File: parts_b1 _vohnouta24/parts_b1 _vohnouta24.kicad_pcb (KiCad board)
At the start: 2 copper layers, 2 parts, among them J1 encoder, J2 SIMSD

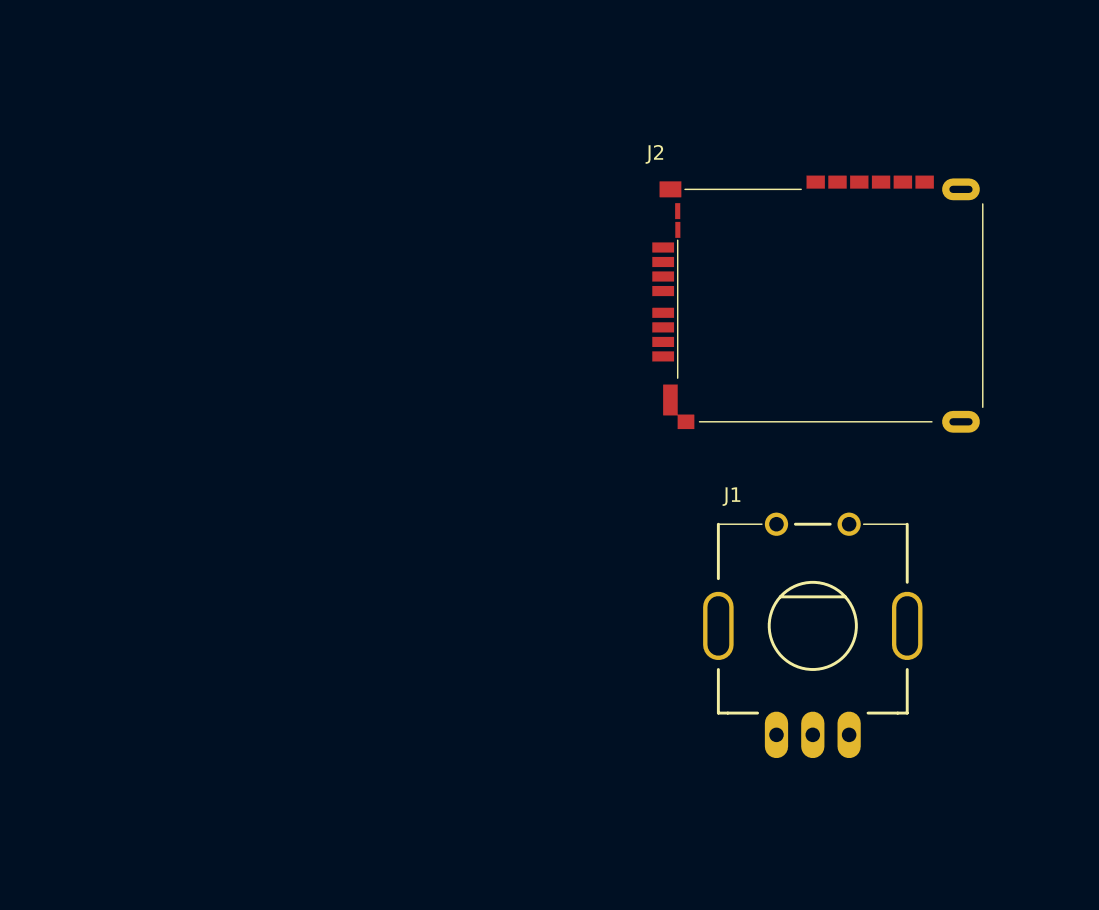
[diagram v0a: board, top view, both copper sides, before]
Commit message: Fix
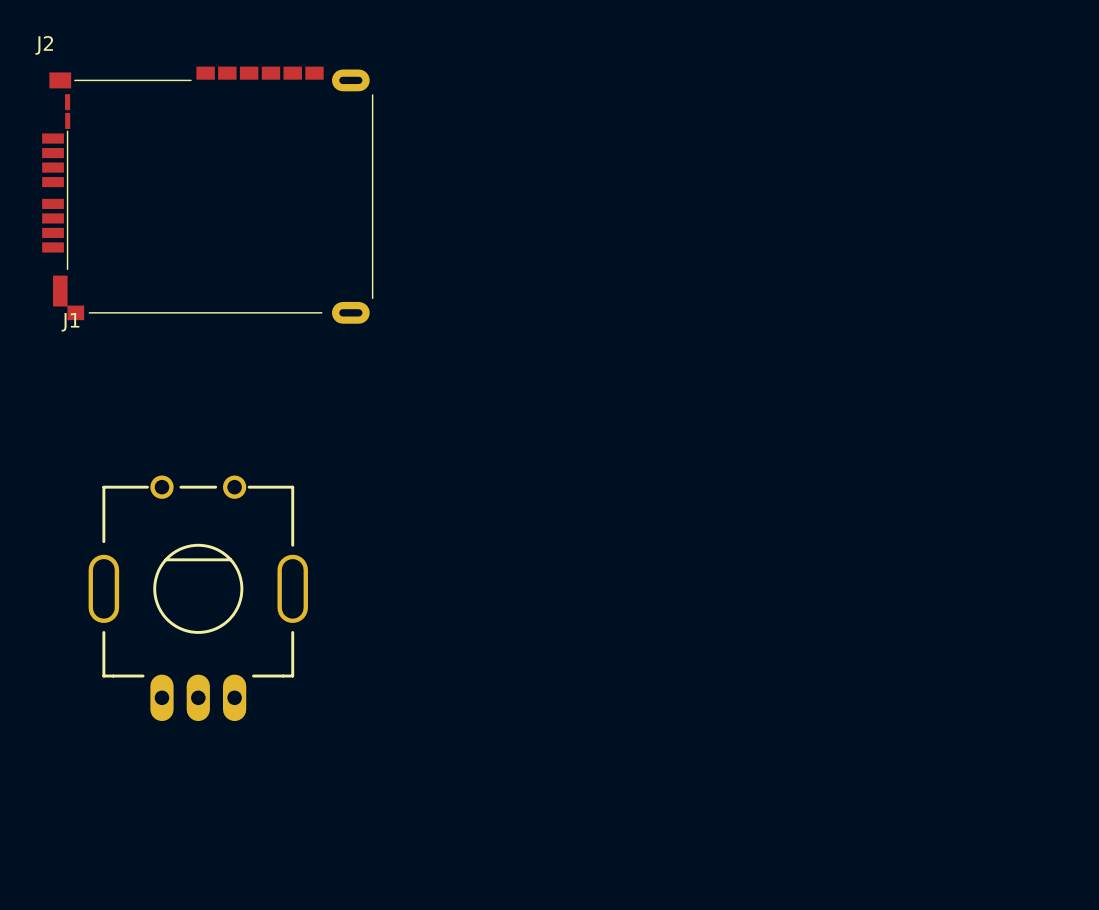
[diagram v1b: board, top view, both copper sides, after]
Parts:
- moved J2 42.7 mm to (127.5, 75.5)
- moved J1 42.4 mm to (129.0, 103.0)
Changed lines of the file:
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@@
 	(footprint "parts_b1_vohnouta24:encoder"
 		(layer "F.Cu")
-		(at 171.3 105.55)
+		(at 129 103)
 		(property "Reference" "J1"
-			(at -5.5 -9 0)
+			(at -8.7 -18.45 0)
 			(unlocked yes)
 			(layer "F.SilkS")
@@
 		)
 		(property "Value" "encoder"
-			(at 4.5 -9 0)
+			(at 1.3 -18.45 0)
 			(unlocked yes)
 			(layer "F.Fab")
@@
 			(end -3.5 -7)
 			(stroke
-				(width 0.1)
-				(type default)
+				(width 0.2)
+				(type solid)
 			)
 			(layer "F.SilkS")
@@
 			(end 3.5 -7)
 			(stroke
-				(width 0.1)
-				(type default)
+				(width 0.2)
+				(type solid)
 			)
 			(layer "F.SilkS")
@@
 	(footprint "parts_b1_vohnouta24:SIMSD"
 		(layer "F.Cu")
-		(at 169.5 83)
+		(at 127.5 75.5)
 		(property "Reference" "J2"
 			(at -9 -10 0)

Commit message: bub fix (yes)
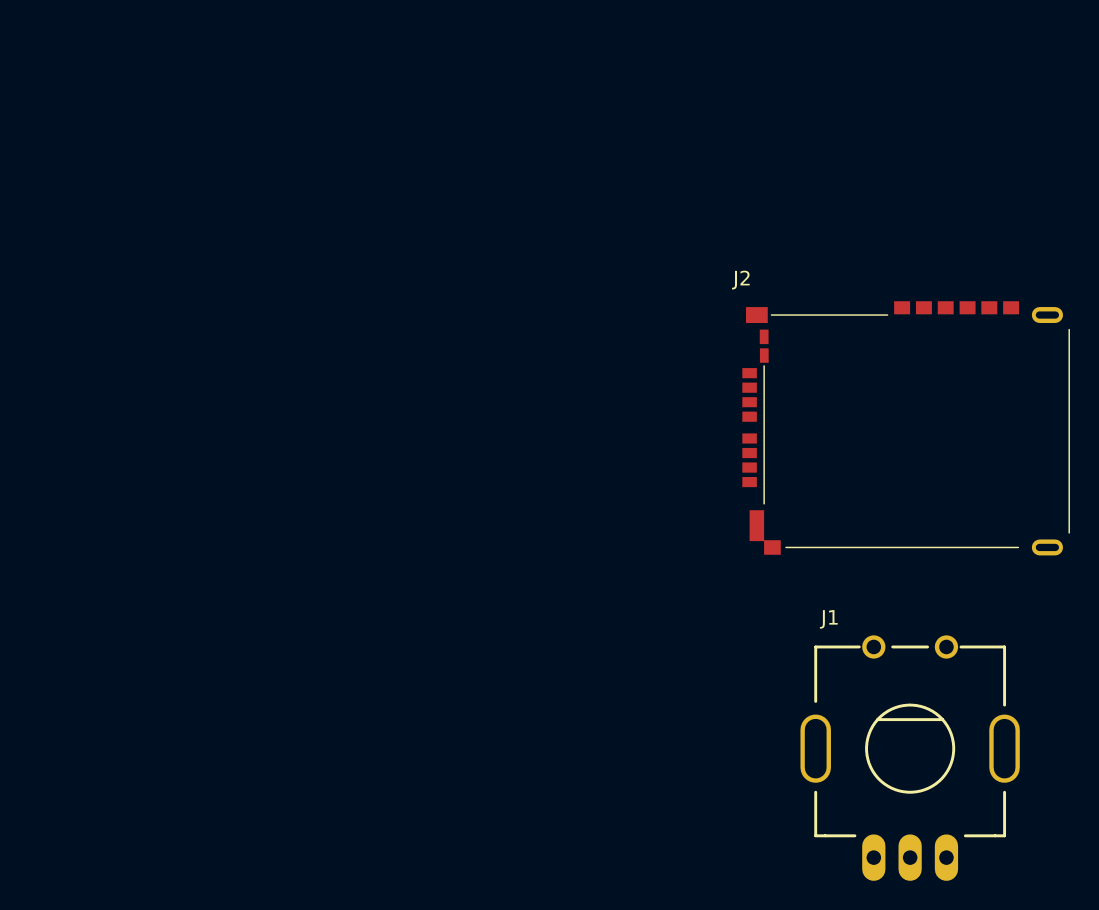
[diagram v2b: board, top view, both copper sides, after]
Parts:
- moved J2 50.6 mm to (175.4, 91.7)
- moved J1 50.2 mm to (178.0, 114.0)
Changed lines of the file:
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@@
 	)
 	(net 0 "")
-	(net 1 "unconnected-(J1-C-Pad3)")
-	(net 2 "unconnected-(J1-A-Pad1)")
+	(net 1 "unconnected-(J1-A-Pad1)")
+	(net 2 "unconnected-(J1-C-Pad3)")
 	(net 3 "unconnected-(J1-B-Pad2)")
-	(net 4 "unconnected-(J2-DAT1-Pad8)")
-	(net 5 "unconnected-(J2-VSS-Pad6)")
-	(net 6 "unconnected-(J2-VCC-Pad11)")
-	(net 7 "unconnected-(J2-DAT3-Pad2)")
-	(net 8 "unconnected-(J2-IO-Pad16)")
-	(net 9 "unconnected-(J2-GND-Pad14)")
+	(net 4 "unconnected-(J2-IO-Pad16)")
+	(net 5 "unconnected-(J2-SWITCHA-Pad9)")
+	(net 6 "unconnected-(J2-DAT2-Pad1)")
+	(net 7 "unconnected-(J2-VSS-Pad6)")
+	(net 8 "unconnected-(J2-RST-Pad12)")
+	(net 9 "unconnected-(J2-CLK-Pad13)")
 	(net 10 "unconnected-(J2-CLK-Pad5)")
-	(net 11 "unconnected-(J2-VPP-Pad15)")
-	(net 12 "unconnected-(J2-CLK-Pad13)")
-	(net 13 "unconnected-(J2-DAT2-Pad1)")
-	(net 14 "unconnected-(J2-SWITCHA-Pad9)")
-	(net 15 "unconnected-(J2-VDD-Pad4)")
-	(net 16 "unconnected-(J2-CMD-Pad3)")
-	(net 17 "unconnected-(J2-SWITCHB-Pad10)")
-	(net 18 "unconnected-(J2-DAT0-Pad7)")
-	(net 19 "unconnected-(J2-RST-Pad12)")
+	(net 11 "unconnected-(J2-DAT0-Pad7)")
+	(net 12 "unconnected-(J2-VCC-Pad11)")
+	(net 13 "unconnected-(J2-CMD-Pad3)")
+	(net 14 "unconnected-(J2-DAT3-Pad2)")
+	(net 15 "unconnected-(J2-GND-Pad14)")
+	(net 16 "unconnected-(J2-SWITCHB-Pad10)")
+	(net 17 "unconnected-(J2-VPP-Pad15)")
+	(net 18 "unconnected-(J2-VDD-Pad4)")
+	(net 19 "unconnected-(J2-DAT1-Pad8)")
 	(footprint "parts_b1_vohnouta24:encoder"
 		(layer "F.Cu")
-		(at 129 103)
+		(at 178 114)
 		(property "Reference" "J1"
-			(at -8.7 -18.45 0)
+			(at -5.5 -9 0)
 			(unlocked yes)
 			(layer "F.SilkS")
@@
 		)
 		(property "Value" "encoder"
-			(at 1.3 -18.45 0)
+			(at 4.5 -9 0)
 			(unlocked yes)
 			(layer "F.Fab")
@@
 			(layers "*.Cu" "*.Mask")
 			(remove_unused_layers no)
-			(net 2 "unconnected-(J1-A-Pad1)")
+			(net 1 "unconnected-(J1-A-Pad1)")
 			(pinfunction "A")
 			(pintype "passive")
@@
 			(layers "*.Cu" "*.Mask")
 			(remove_unused_layers no)
-			(net 1 "unconnected-(J1-C-Pad3)")
+			(net 2 "unconnected-(J1-C-Pad3)")
 			(pinfunction "C")
 			(pintype "passive")
@@
 	(footprint "parts_b1_vohnouta24:SIMSD"
 		(layer "F.Cu")
-		(at 127.5 75.5)
+		(at 175.45 91.65)
 		(property "Reference" "J2"
 			(at -9 -10 0)
@@
 		)
 		(property "Value" "SIMSD"
-			(at -7.5 11 0)
+			(at -3.5 15.5 0)
 			(unlocked yes)
 			(layer "F.Fab")
@@
 			(layer "F.SilkS")
 		)
+		(pad "" smd rect
+			(at -8 -7.5)
+			(size 1.5 1.1)
+			(layers "F.Cu" "F.Mask" "F.Paste")
+		)
+		(pad "" smd rect
+			(at -8 7)
+			(size 1 2.13)
+			(layers "F.Cu" "F.Mask" "F.Paste")
+		)
+		(pad "" smd rect
+			(at -6.93 8.5)
+			(size 1.15 1)
+			(layers "F.Cu" "F.Mask" "F.Paste")
+		)
+		(pad "" thru_hole oval
+			(at 12 -7.5)
+			(size 2.15 1.1)
+			(drill oval 1.6 0.5)
+			(layers "*.Cu" "*.Mask")
+			(remove_unused_layers no)
+		)
+		(pad "" thru_hole oval
+			(at 12 8.5)
+			(size 2.15 1.1)
+			(drill oval 1.6 0.5)
+			(layers "*.Cu" "*.Mask")
+			(remove_unused_layers no)
+		)
 		(pad "1" smd rect
 			(at -8.5 -3.5 180)
-			(size 1.5 0.7)
-			(layers "F.Cu" "F.Mask" "F.Paste")
-			(net 13 "unconnected-(J2-DAT2-Pad1)")
+			(size 1 0.7)
+			(layers "F.Cu" "F.Mask" "F.Paste")
+			(net 6 "unconnected-(J2-DAT2-Pad1)")
 			(pinfunction "DAT2")
 			(pintype "bidirectional")
@@
 		(pad "2" smd rect
 			(at -8.5 -2.5 180)
-			(size 1.5 0.7)
-			(layers "F.Cu" "F.Mask" "F.Paste")
-			(net 7 "unconnected-(J2-DAT3-Pad2)")
+			(size 1 0.7)
+			(layers "F.Cu" "F.Mask" "F.Paste")
+			(net 14 "unconnected-(J2-DAT3-Pad2)")
 			(pinfunction "DAT3")
 			(pintype "bidirectional")
@@
 		(pad "3" smd rect
 			(at -8.5 -1.5 180)
-			(size 1.5 0.7)
-			(layers "F.Cu" "F.Mask" "F.Paste")
-			(net 16 "unconnected-(J2-CMD-Pad3)")
+			(size 1 0.7)
+			(layers "F.Cu" "F.Mask" "F.Paste")
+			(net 13 "unconnected-(J2-CMD-Pad3)")
 			(pinfunction "CMD")
 			(pintype "bidirectional")
@@
 		(pad "4" smd rect
 			(at -8.5 -0.5 180)
-			(size 1.5 0.7)
-			(layers "F.Cu" "F.Mask" "F.Paste")
-			(net 15 "unconnected-(J2-VDD-Pad4)")
+			(size 1 0.7)
+			(layers "F.Cu" "F.Mask" "F.Paste")
+			(net 18 "unconnected-(J2-VDD-Pad4)")
 			(pinfunction "VDD")
 			(pintype "power_in")
@@
 		(pad "5" smd rect
 			(at -8.5 1 180)
-			(size 1.5 0.7)
+			(size 1 0.7)
 			(layers "F.Cu" "F.Mask" "F.Paste")
 			(net 10 "unconnected-(J2-CLK-Pad5)")
@@
 		(pad "6" smd rect
 			(at -8.5 2 180)
-			(size 1.5 0.7)
-			(layers "F.Cu" "F.Mask" "F.Paste")
-			(net 5 "unconnected-(J2-VSS-Pad6)")
+			(size 1 0.7)
+			(layers "F.Cu" "F.Mask" "F.Paste")
+			(net 7 "unconnected-(J2-VSS-Pad6)")
 			(pinfunction "VSS")
 			(pintype "power_in")
@@
 		(pad "7" smd rect
 			(at -8.5 3 180)
-			(size 1.5 0.7)
-			(layers "F.Cu" "F.Mask" "F.Paste")
-			(net 18 "unconnected-(J2-DAT0-Pad7)")
+			(size 1 0.7)
+			(layers "F.Cu" "F.Mask" "F.Paste")
+			(net 11 "unconnected-(J2-DAT0-Pad7)")
 			(pinfunction "DAT0")
 			(pintype "bidirectional")
@@
 		(pad "8" smd rect
 			(at -8.5 4 180)
-			(size 1.5 0.7)
-			(layers "F.Cu" "F.Mask" "F.Paste")
-			(net 4 "unconnected-(J2-DAT1-Pad8)")
+			(size 1 0.7)
+			(layers "F.Cu" "F.Mask" "F.Paste")
+			(net 19 "unconnected-(J2-DAT1-Pad8)")
 			(pinfunction "DAT1")
 			(pintype "bidirectional")
@@
 		(pad "9" smd rect
 			(at -7.5 -6 270)
-			(size 1.1 0.35)
-			(layers "F.Cu" "F.Mask" "F.Paste")
-			(net 14 "unconnected-(J2-SWITCHA-Pad9)")
+			(size 1 0.6)
+			(layers "F.Cu" "F.Mask" "F.Paste")
+			(net 5 "unconnected-(J2-SWITCHA-Pad9)")
 			(pinfunction "SWITCHA")
 			(pintype "passive")
@@
 		(pad "10" smd rect
 			(at -7.49 -4.71 270)
-			(size 1.1 0.35)
-			(layers "F.Cu" "F.Mask" "F.Paste")
-			(net 17 "unconnected-(J2-SWITCHB-Pad10)")
+			(size 1 0.6)
+			(layers "F.Cu" "F.Mask" "F.Paste")
+			(net 16 "unconnected-(J2-SWITCHB-Pad10)")
 			(pinfunction "SWITCHB")
 			(pintype "passive")
@@
 		(pad "11" smd rect
 			(at 9.5 -8 270)
-			(size 0.9 1.27)
-			(layers "F.Cu" "F.Mask" "F.Paste")
-			(net 6 "unconnected-(J2-VCC-Pad11)")
+			(size 0.9 1.1)
+			(layers "F.Cu" "F.Mask" "F.Paste")
+			(net 12 "unconnected-(J2-VCC-Pad11)")
 			(pinfunction "VCC")
 			(pintype "power_in")
@@
 		(pad "12" smd rect
 			(at 6.5 -8 270)
-			(size 0.9 1.27)
-			(layers "F.Cu" "F.Mask" "F.Paste")
-			(net 19 "unconnected-(J2-RST-Pad12)")
+			(size 0.9 1.1)
+			(layers "F.Cu" "F.Mask" "F.Paste")
+			(net 8 "unconnected-(J2-RST-Pad12)")
 			(pinfunction "RST")
 			(pintype "bidirectional")
@@
 		(pad "13" smd rect
 			(at 3.5 -8 270)
-			(size 0.9 1.27)
-			(layers "F.Cu" "F.Mask" "F.Paste")
-			(net 12 "unconnected-(J2-CLK-Pad13)")
+			(size 0.9 1.1)
+			(layers "F.Cu" "F.Mask" "F.Paste")
+			(net 9 "unconnected-(J2-CLK-Pad13)")
 			(pinfunction "CLK")
 			(pintype "bidirectional")
@@
 		(pad "14" smd rect
 			(at 8 -8 270)
-			(size 0.9 1.27)
-			(layers "F.Cu" "F.Mask" "F.Paste")
-			(net 9 "unconnected-(J2-GND-Pad14)")
+			(size 0.9 1.1)
+			(layers "F.Cu" "F.Mask" "F.Paste")
+			(net 15 "unconnected-(J2-GND-Pad14)")
 			(pinfunction "GND")
 			(pintype "power_in")
@@
 		(pad "15" smd rect
 			(at 5 -8 270)
-			(size 0.9 1.27)
-			(layers "F.Cu" "F.Mask" "F.Paste")
-			(net 11 "unconnected-(J2-VPP-Pad15)")
+			(size 0.9 1.1)
+			(layers "F.Cu" "F.Mask" "F.Paste")
+			(net 17 "unconnected-(J2-VPP-Pad15)")
 			(pinfunction "VPP")
 			(pintype "bidirectional")
@@
 		(pad "16" smd rect
 			(at 2 -8 270)
-			(size 0.9 1.27)
-			(layers "F.Cu" "F.Mask" "F.Paste")
-			(net 8 "unconnected-(J2-IO-Pad16)")
+			(size 0.9 1.1)
+			(layers "F.Cu" "F.Mask" "F.Paste")
+			(net 4 "unconnected-(J2-IO-Pad16)")
 			(pinfunction "IO")
 			(pintype "bidirectional")
 		)
-		(pad "SH" smd rect
-			(at -8 -7.5)
-			(size 1.5 1.1)
-			(layers "F.Cu" "F.Mask" "F.Paste")
-		)
-		(pad "SH" smd rect
-			(at -8 7)
-			(size 1 2.13)
-			(layers "F.Cu" "F.Mask" "F.Paste")
-		)
-		(pad "SH" smd rect
-			(at -6.93 8.5)
-			(size 1.15 1)
-			(layers "F.Cu" "F.Mask" "F.Paste")
-		)
-		(pad "SH" thru_hole oval
-			(at 12 -7.5)
-			(size 2.6 1.5)
-			(drill oval 1.6 0.5)
-			(layers "*.Cu" "*.Mask")
-			(remove_unused_layers no)
-		)
-		(pad "SH" thru_hole oval
-			(at 12 8.5)
-			(size 2.6 1.5)
-			(drill oval 1.6 0.5)
-			(layers "*.Cu" "*.Mask")
-			(remove_unused_layers no)
-		)
 		(embedded_fonts no)
